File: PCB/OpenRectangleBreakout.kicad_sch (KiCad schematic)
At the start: 43 parts, among them J1 USB C Connector, J2 JTAG_TC2030, J3 Conn_01x04_Pin, J4 Conn_01x04_Pin, J5 Conn_01x06_Pin, SW1 Boot, U1 XC6206, U2 USBLC6-2SC6, U3 RP2040, U4 W25Q128JVS, Y1 12MHz

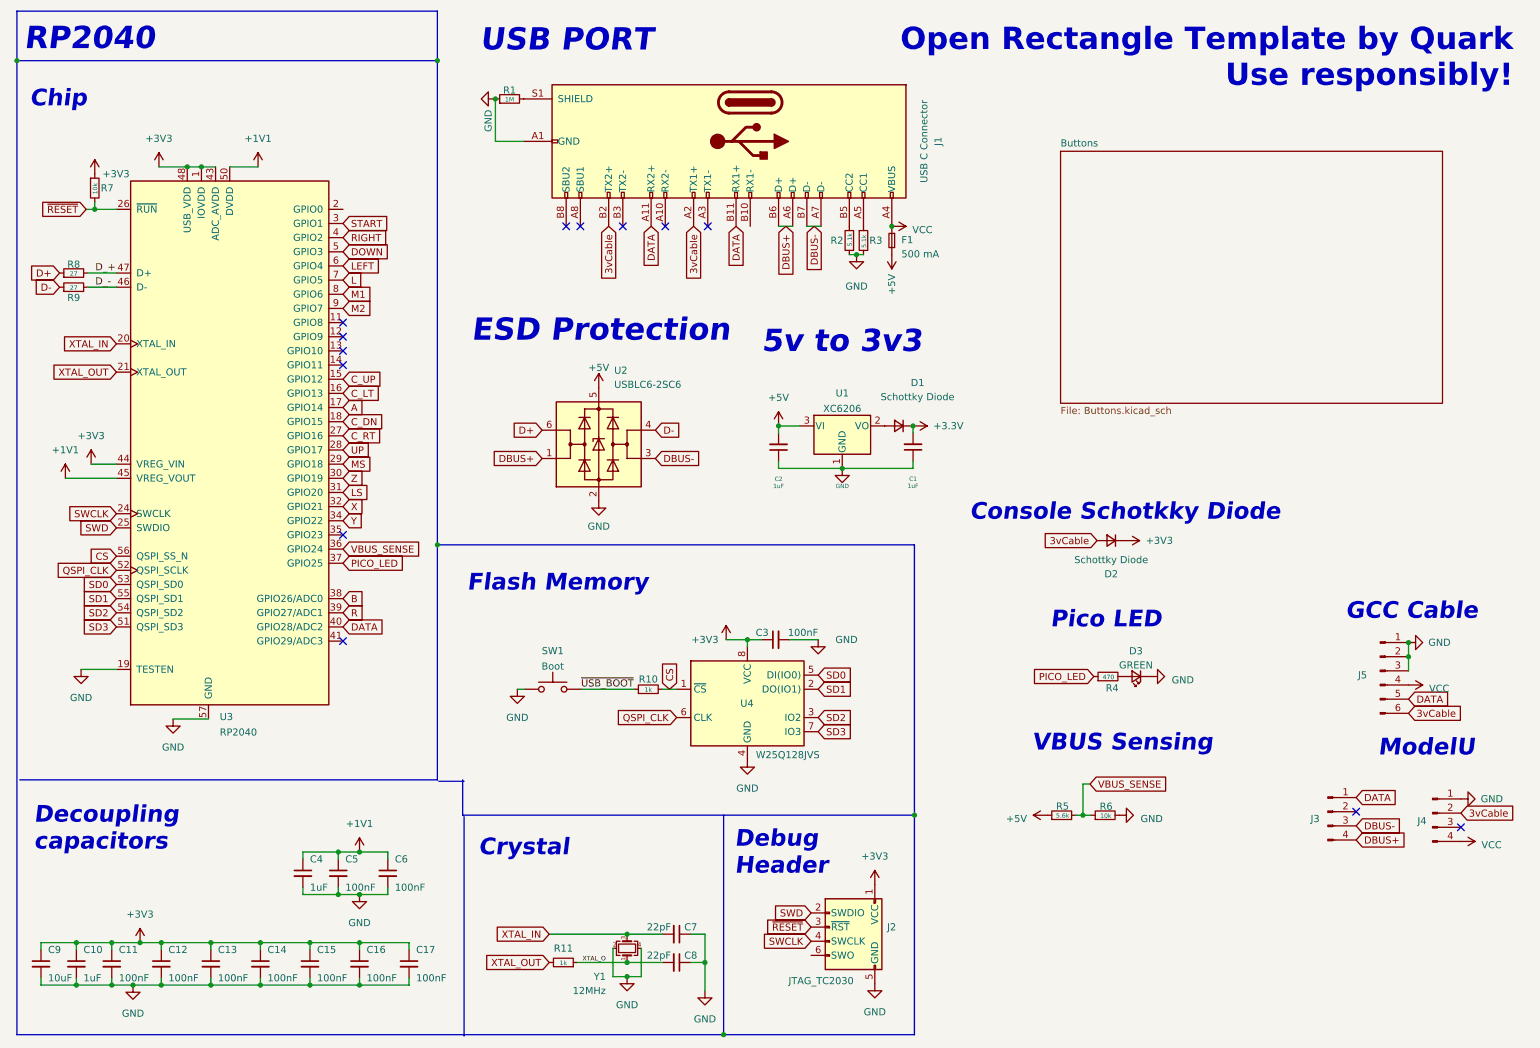
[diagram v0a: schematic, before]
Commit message: First version
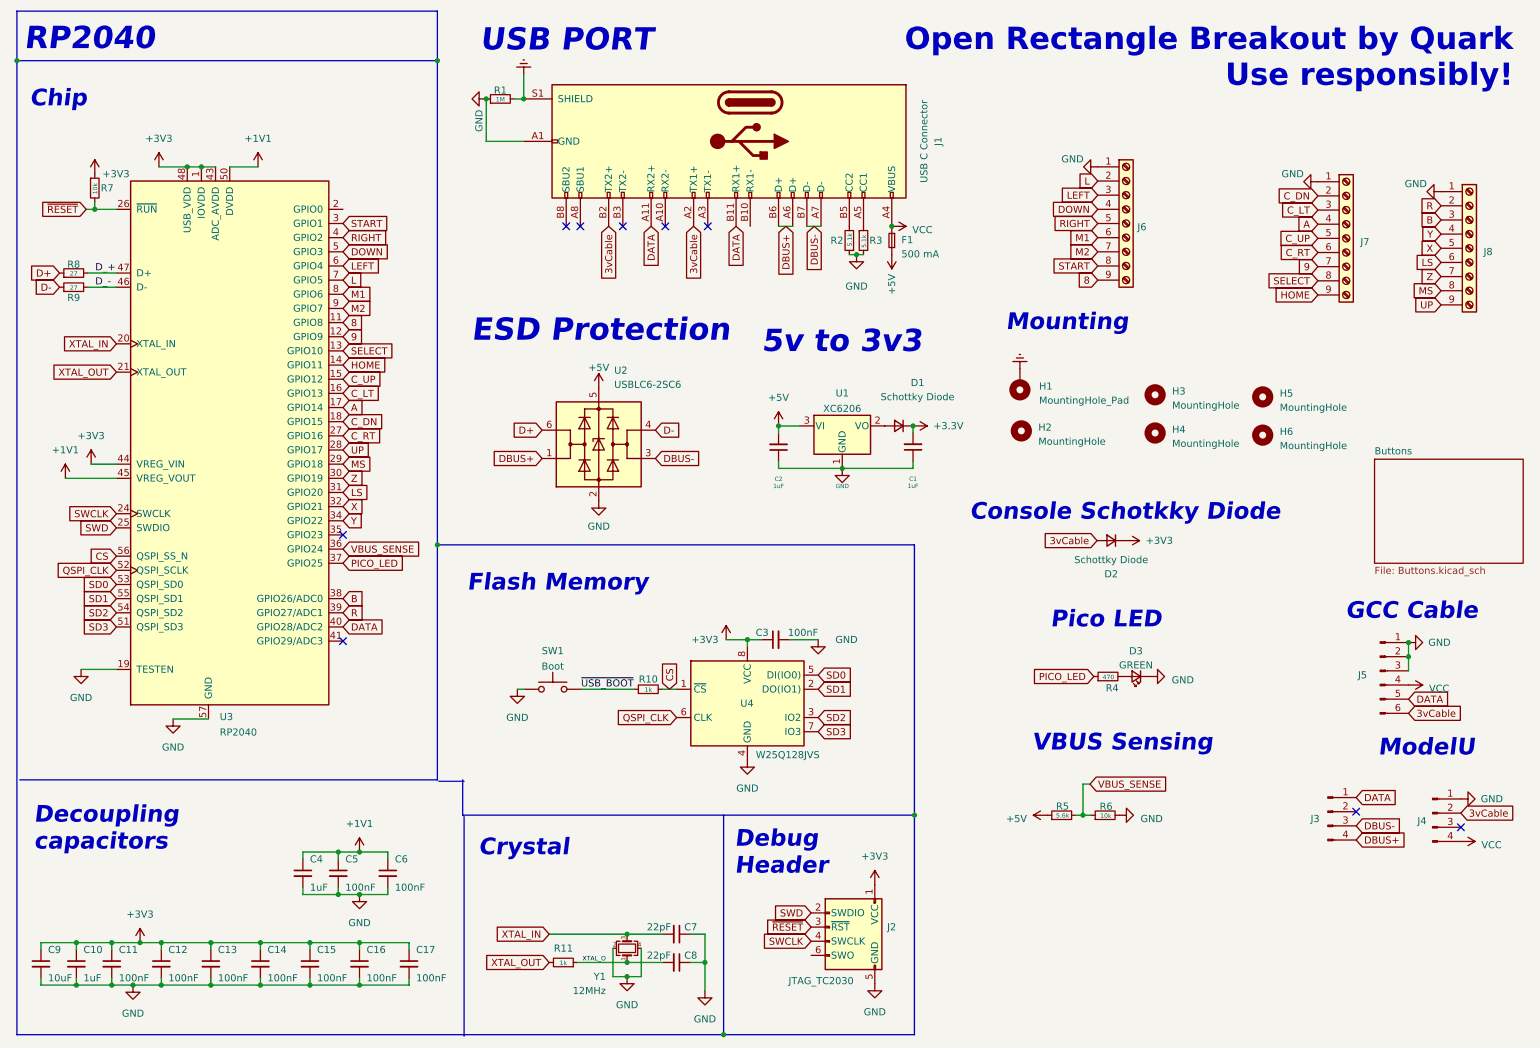
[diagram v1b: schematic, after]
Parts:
- added H1: MountingHole_Pad, MountingHole:MountingHole_2.2mm_M2_ISO14580_Pad, symbol Mechanical:MountingHole_Pad
- added H2, H3, H4, H5, H6: MountingHole, MountingHole:MountingHole_2.1mm, symbol Mechanical:MountingHole
- added J6, J7, J8: Screw_Terminal_01x09, Connector_PinHeader_2.54mm:PinHeader_1x09_P2.54mm_Vertical, symbol Connector:Screw_Terminal_01x09
- D3: LCSC (none) -> C2297
- J5: value Conn_01x06_Pin -> GCC Cable; footprint Connector_PinHeader_2.54mm:PinHeader_1x06_P2.54mm_Vertical -> Connector_PinHeader_2.00mm:PinHeader_1x06_P2.00mm_Vertical
- R4: LCSC (none) -> C25117
- R5, R6: footprint Resistor_SMD:R_0603_1608Metric -> Resistor_SMD:R_0402_1005Metric
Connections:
- net A: now also J7.4 (Pin_4)
- net B: now also J8.3 (Pin_3)
- net C_DN: now also J7.2 (Pin_2)
- net C_LT: now also J7.3 (Pin_3)
- net C_RT: now also J7.6 (Pin_6)
- net C_UP: now also J7.5 (Pin_5)
- net DOWN: now also J6.4 (Pin_4)
- net GND: now also J6.1 (Pin_1), J7.1 (Pin_1), J8.1 (Pin_1)
- net L: now also J6.2 (Pin_2)
- net LEFT: now also J6.3 (Pin_3)
- net LS: now also J8.6 (Pin_6)
- net M1: now also J6.6 (Pin_6)
- net M2: now also J6.7 (Pin_7)
- net MS: now also J8.8 (Pin_8)
- net R: now also J8.2 (Pin_2)
- net RIGHT: now also J6.5 (Pin_5)
- net START: now also J6.8 (Pin_8)
- net UP: now also J8.9 (Pin_9)
- net X: now also J8.5 (Pin_5)
- net Y: now also J8.4 (Pin_4)
- net Z: now also J8.7 (Pin_7)
- net 8: now reaches U3.11 (GPIO8)
- net 8: now also J6.9 (Pin_9)
- net 9: now reaches U3.12 (GPIO9)
- net 9: now also J7.7 (Pin_7)
- net SELECT: now reaches U3.13 (GPIO10)
- net SELECT: now also J7.8 (Pin_8)
- net HOME: now reaches U3.14 (GPIO11)
- net HOME: now also J7.9 (Pin_9)
- net Earth: now reaches J1.S1 (SHIELD), R1.2
- net Earth: now also H1.1
- no-connect marks 13 -> 9
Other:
- note added: "Mounting"
- note added: "Open Rectangle Breakout by Quark Use responsibly!"
- note removed: "Open Rectangle Template by Quark Use responsibly!"
- moved on the sheet: R1
